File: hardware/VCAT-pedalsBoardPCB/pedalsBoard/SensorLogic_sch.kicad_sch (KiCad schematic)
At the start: 13 parts, among them U4 Opamp_Dual, U5 Opamp_Dual

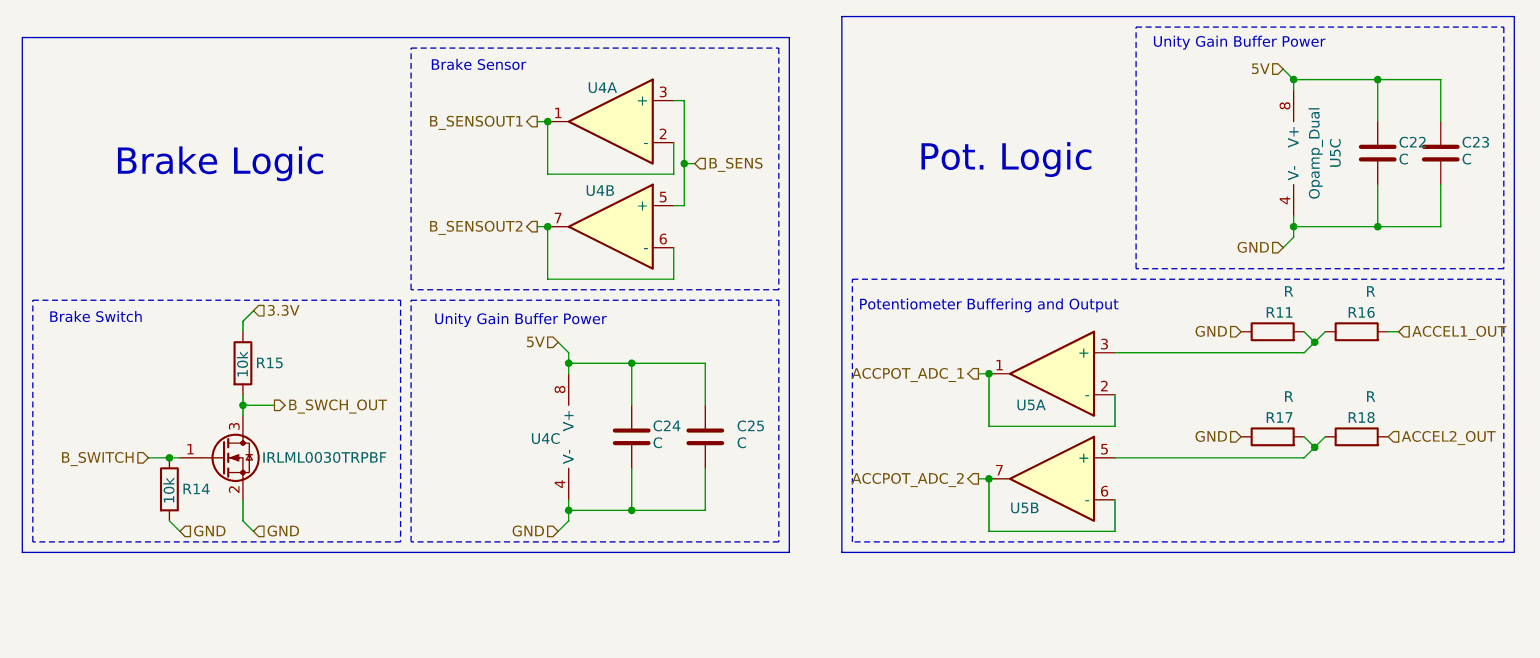
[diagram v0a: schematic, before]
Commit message: test
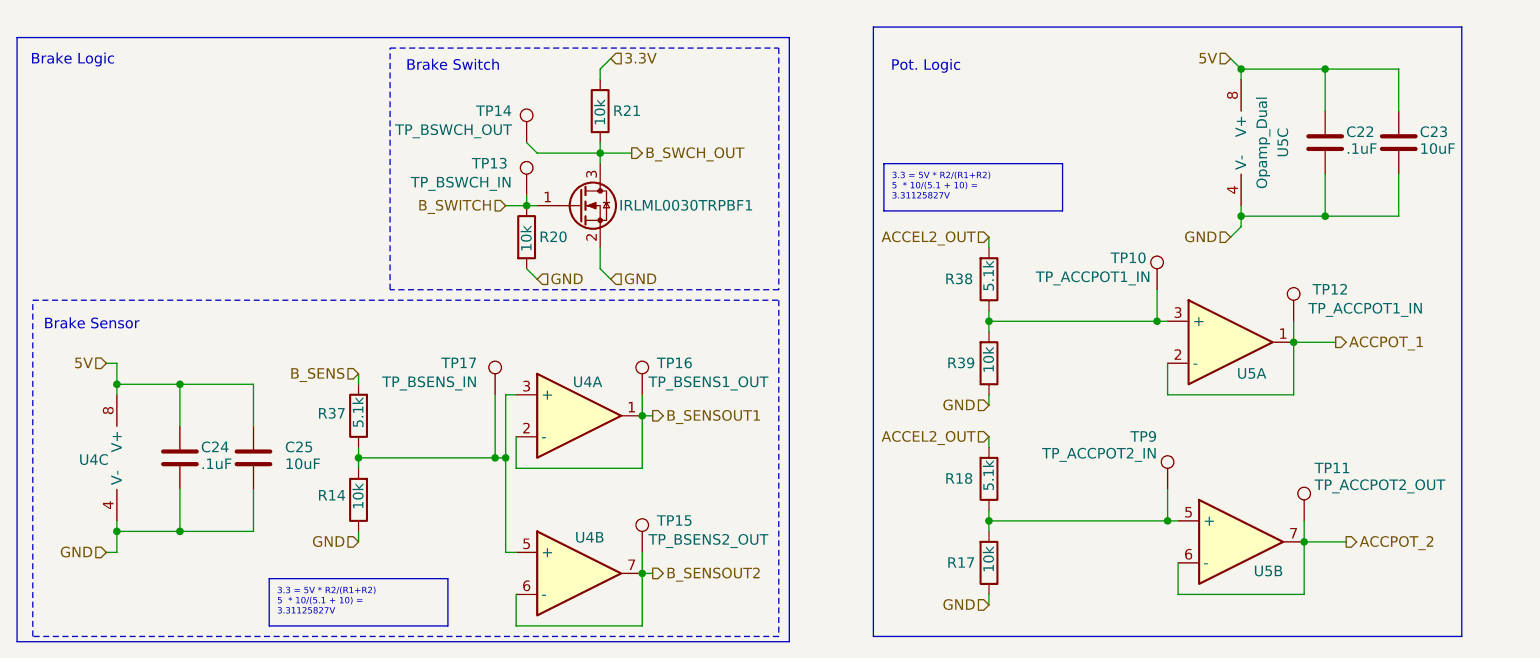
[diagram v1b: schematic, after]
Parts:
- removed IRLML0030TRPBF: IRLML0030, SOT95P237X112-3N, symbol Transistor_FET:IRLML0030
- removed R11, R16: R, symbol Device:R
- removed R15: 10k, symbol Device:R
- added IRLML0030TRPBF1: IRLML0030, SOT95P237X112-3N, symbol Transistor_FET:IRLML0030
- added R20, R21, R39: 10k, Resistor_SMD:R_0603_1608Metric_Pad0.98x0.95mm_HandSolder, symbol Device:R
- added R37, R38: 5.1k, Resistor_SMD:R_0603_1608Metric_Pad0.98x0.95mm_HandSolder, symbol Device:R
- added TP10, TP12: TP_ACCPOT1_IN, symbol Connector:TestPoint
- added TP11: TP_ACCPOT2_OUT, symbol Connector:TestPoint
- added TP13: TP_BSWCH_IN, symbol Connector:TestPoint
- added TP14: TP_BSWCH_OUT, symbol Connector:TestPoint
- added TP15: TP_BSENS2_OUT, symbol Connector:TestPoint
- added TP16: TP_BSENS1_OUT, symbol Connector:TestPoint
- added TP17: TP_BSENS_IN, symbol Connector:TestPoint
- added TP9: TP_ACCPOT2_IN, symbol Connector:TestPoint
- C22, C24: value C -> .1uF; footprint (none) -> Capacitor_SMD:C_0603_1608Metric_Pad1.08x0.95mm_HandSolder
- C23, C25: value C -> 10uF; footprint (none) -> Capacitor_SMD:C_0603_1608Metric_Pad1.08x0.95mm_HandSolder
- R14: footprint (none) -> Resistor_SMD:R_0603_1608Metric_Pad0.98x0.95mm_HandSolder
- R17: value R -> 10k; footprint (none) -> Resistor_SMD:R_0603_1608Metric_Pad0.98x0.95mm_HandSolder
- R18: value R -> 5.1k; footprint (none) -> Resistor_SMD:R_0603_1608Metric_Pad0.98x0.95mm_HandSolder
- U4: footprint (none) -> MyParts:SOIC127P600X175-8N
- U5: footprint SOIC127P600X175-8N -> MyParts:SOIC127P600X175-8N
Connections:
- net 3.3V: now also R21.1
- net ACCEL2_OUT: now also R38.2
- net B_SENS: now also R37.2; no longer U4.3 (+), U4.5 (+)
- net B_SENSOUT1: now also TP16.1
- net B_SENSOUT2: now also TP15.1
- net B_SWCH_OUT: now also IRLML0030TRPBF1.3 (D), R21.2, TP14.1
- net B_SWITCH: now also IRLML0030TRPBF1.1 (G), R20.1, TP13.1; no longer R14.1
- net GND: now also R14.1, IRLML0030TRPBF1.2 (S), R20.2, R39.1; no longer R14.2
- net at R17.2, R18.1, U5.5 (+): now also TP9.1
- net at U5.3 (+): now also R38.1, R39.2, TP10.1
- net ACCPOT_ADC_1 renamed ACCPOT_1
- net ACCPOT_1: now also TP12.1
- net ACCPOT_ADC_2 renamed ACCPOT_2
- net ACCPOT_2: now also TP11.1
- new net: R14.2, R37.1, TP17.1, U4.3 (+), U4.5 (+)
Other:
- note removed: "Potentiometer Buffering and Output"
- note removed: "Unity Gain Buffer Power"
- moved on the sheet: C22, C23, C24, C25, R17, R18, U4A, U4B, U4C, U5A, U5B, U5C
